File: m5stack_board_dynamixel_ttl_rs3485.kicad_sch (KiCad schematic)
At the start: 15 parts, among them J2 B2B-XH-A(LF)(SN), J2 WAFER-HY2.0-4PZZ, J4 B3B-EH-A(LF)(SN), Q1 2SA1162GR, U1 MAX3485, U2 AP7333-33SAG

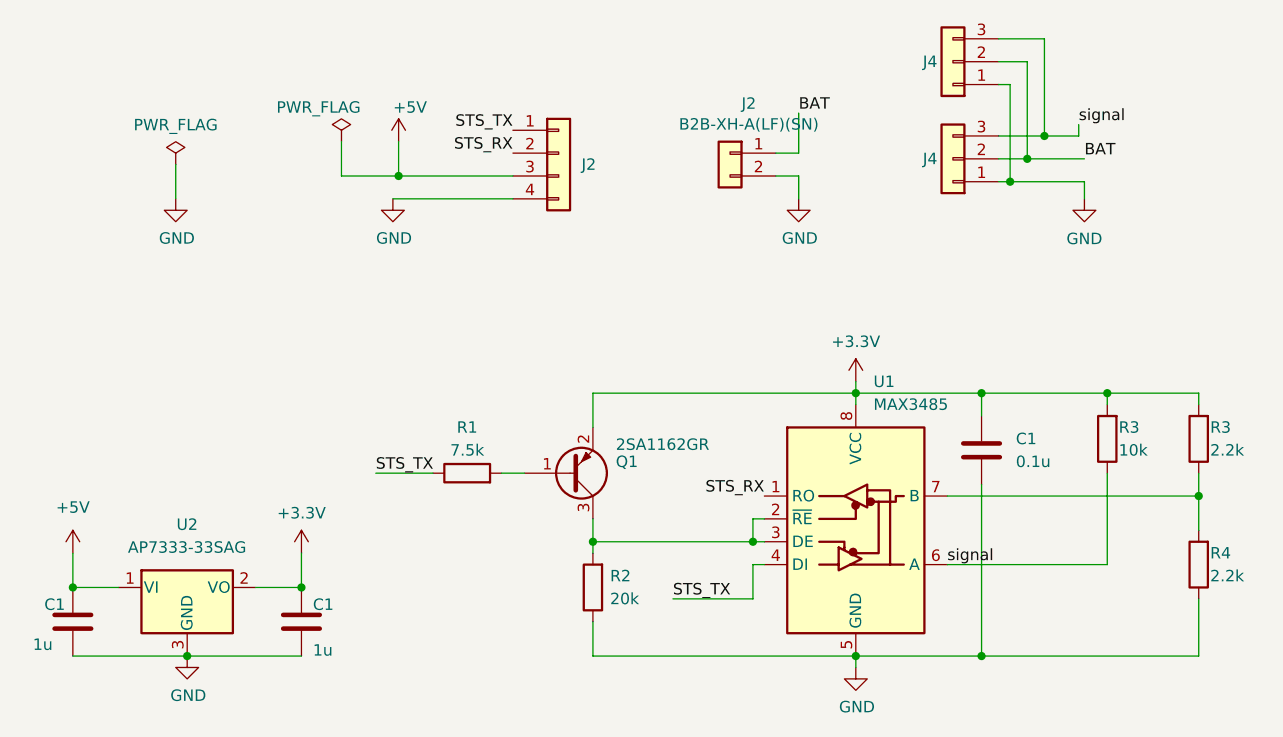
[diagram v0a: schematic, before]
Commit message: update board
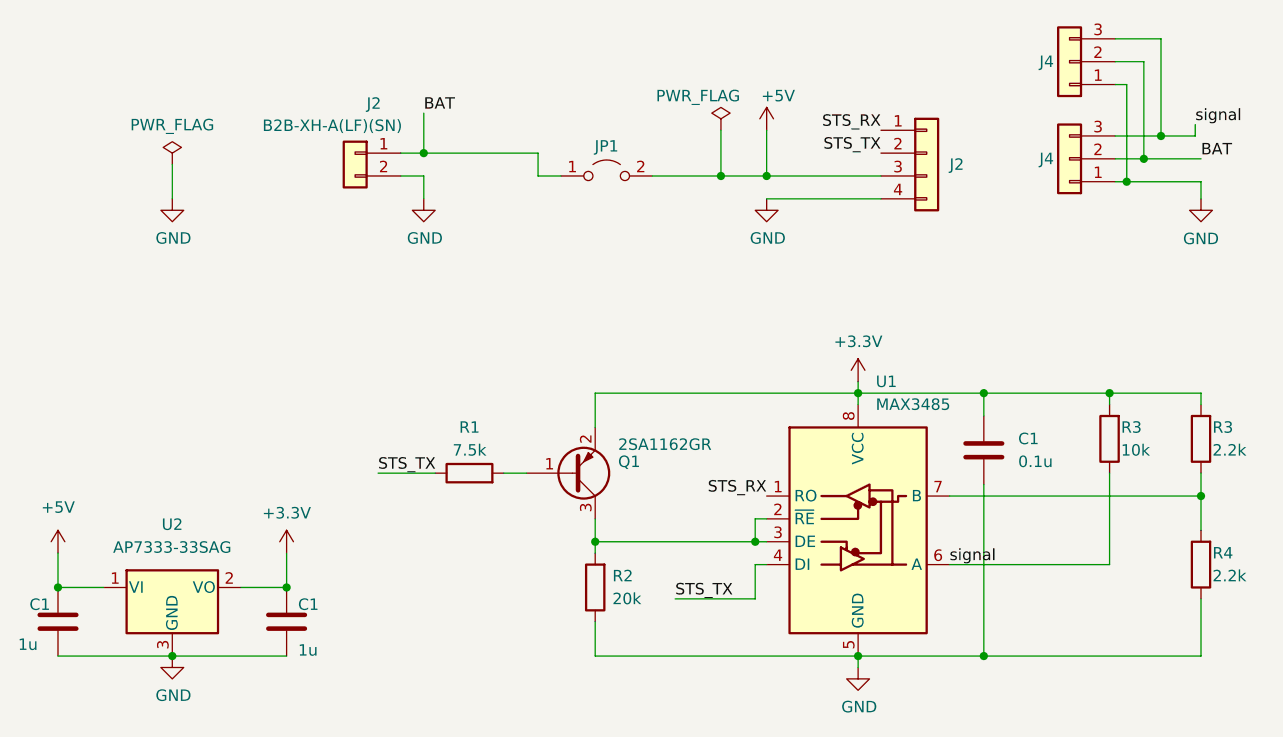
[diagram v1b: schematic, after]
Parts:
- added JP1: Jumper_2_Open, Jumper:SolderJumper-2_P1.3mm_Open_RoundedPad1.0x1.5mm, symbol Jumper:Jumper_2_Open
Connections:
- net +5V: now also JP1.2 (B)
- net BAT: now also JP1.1 (A)
- net STS_RX: now also J2.1 (Pin_1); no longer J2.2 (Pin_2)
- net STS_TX: now also J2.2 (Pin_2); no longer J2.1 (Pin_1)
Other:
- moved on the sheet: C1, J2, J4, U2
